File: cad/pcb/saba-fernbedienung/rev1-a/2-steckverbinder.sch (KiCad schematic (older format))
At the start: 28 parts, among them J301 Conn_01x04, J302 Conn_01x04, J303 Micro_SD_Card, J304 Conn_01x04, J305 AudioJack3_Ground, J306 Conn_01x02, J307 Conn_01x04, J308 Conn_01x01, J309 Conn_01x01, J310 Conn_01x01, J311 Conn_01x04, J312 USB_C_Receptacle_USB2.0, U301 TSOP31238

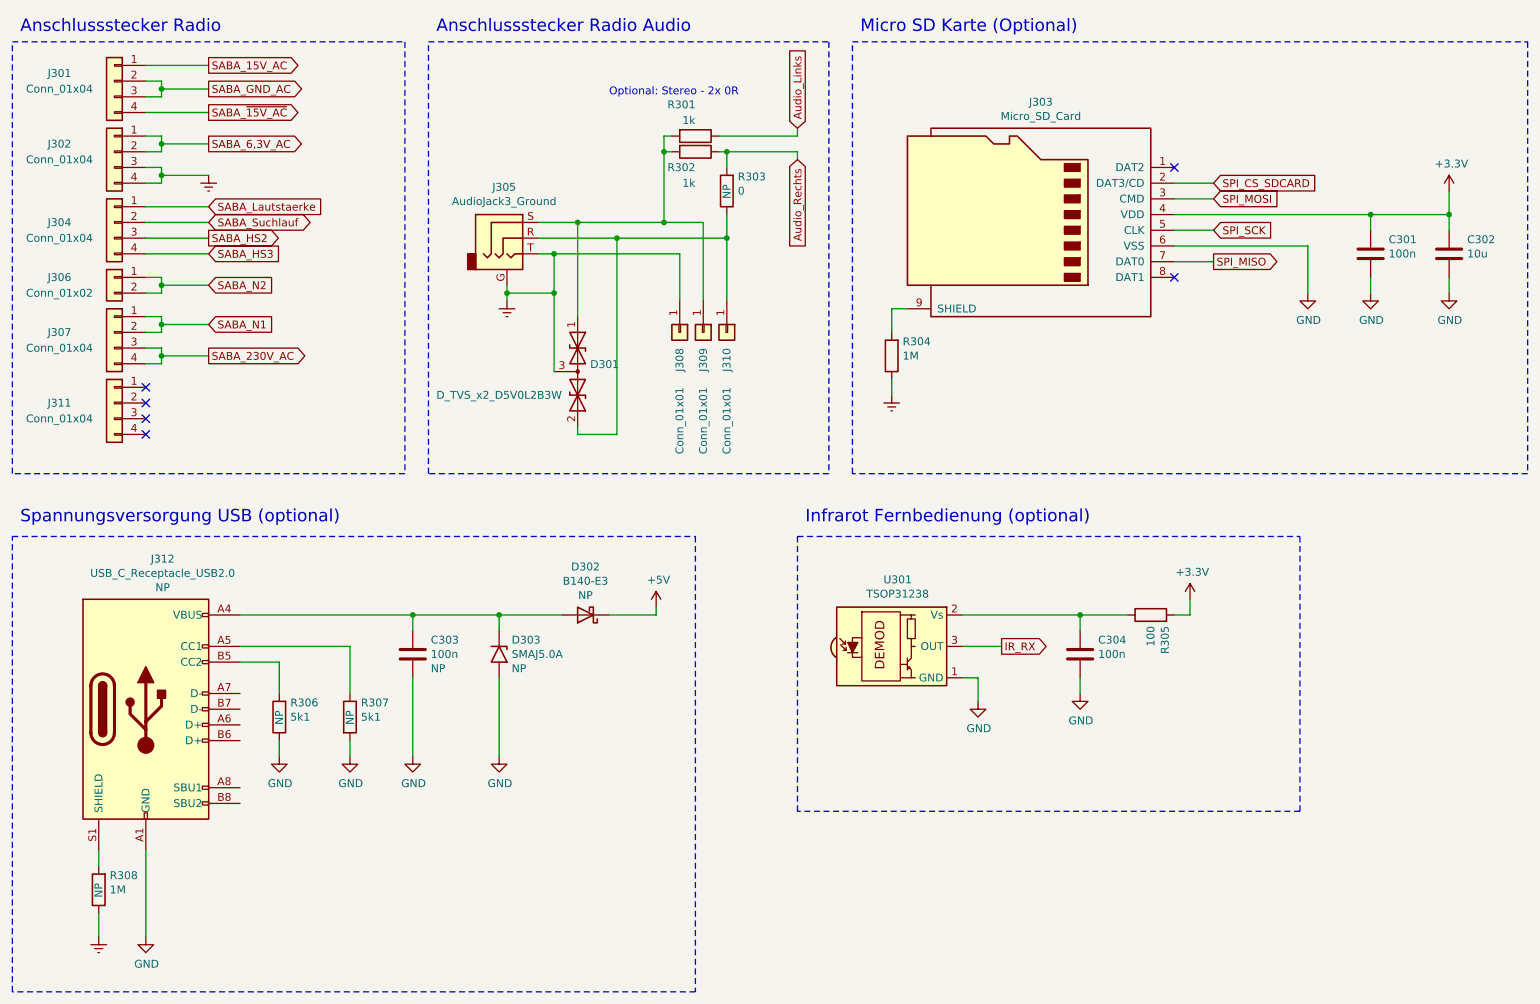
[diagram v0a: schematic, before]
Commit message: Fix: Div. DRC
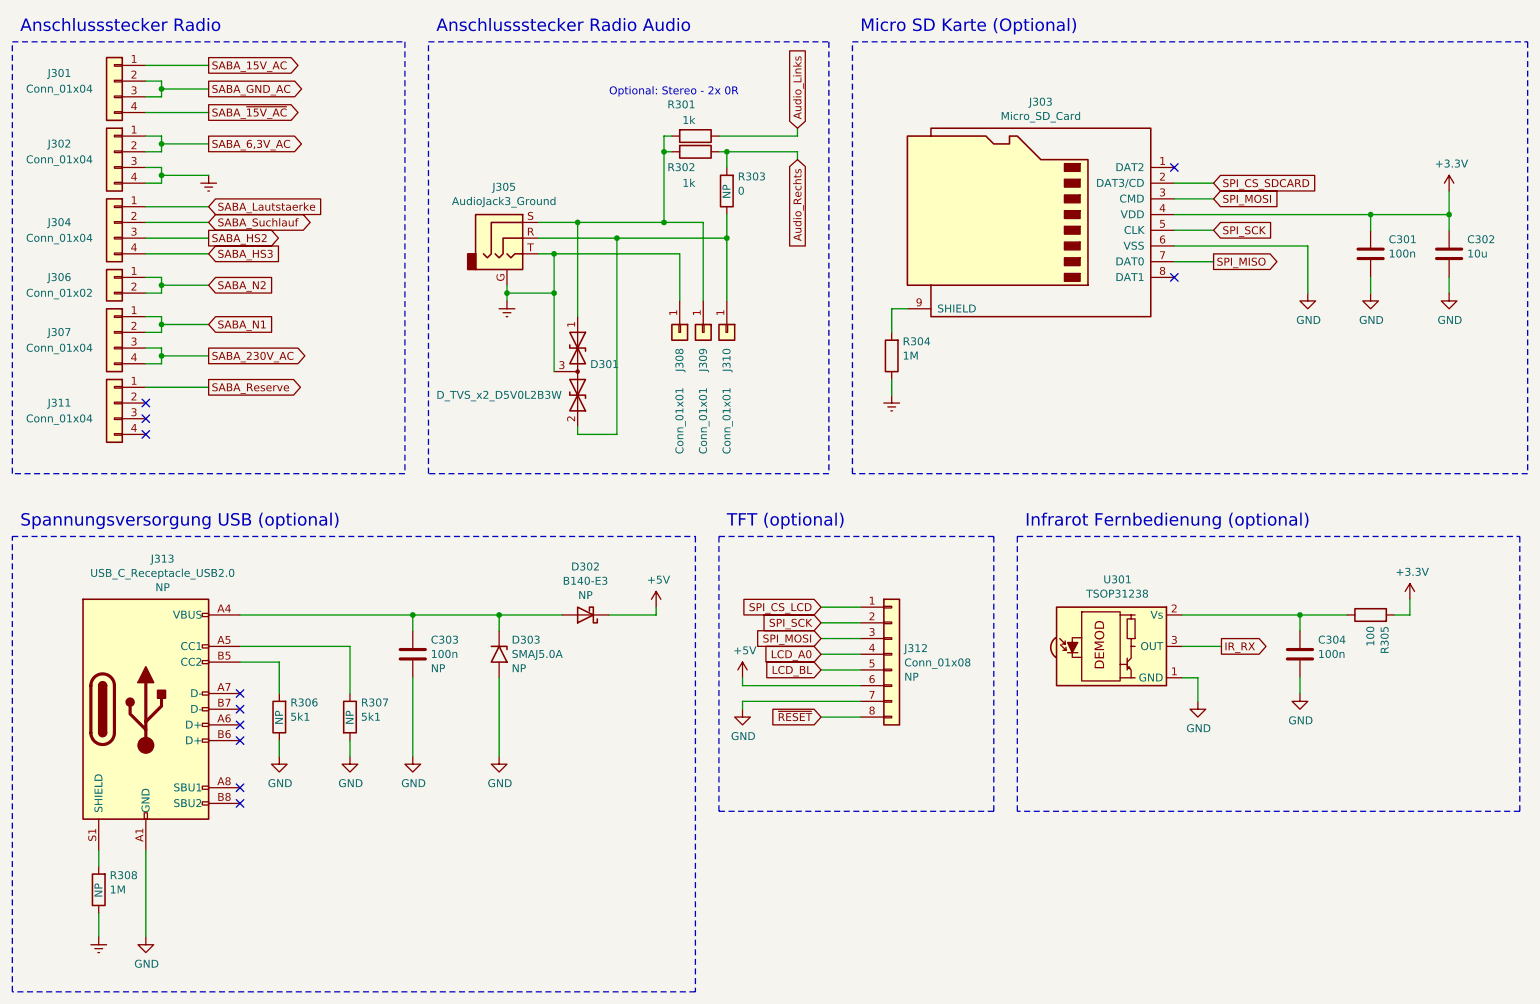
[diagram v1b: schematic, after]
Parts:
- added J312: Conn_01x08, symbol Connector_Generic:Conn_01x08
- renumbered J312 to J313
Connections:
- net +5V: now also J312.6 (Pin_6)
- net GND: now also J312.7 (Pin_7)
- net SPI_MOSI: now also J312.3 (Pin_3)
- net SPI_SCK: now also J312.2 (Pin_2)
- net SABA_Reserve: now reaches J311.1 (Pin_1)
- new net LCD_A0: J312.4 (Pin_4)
- new net LCD_BL: J312.5 (Pin_5)
- new net SPI_CS_LCD: J312.1 (Pin_1)
- new net ~RESET: J312.8 (Pin_8)
- no-connect marks 6 -> 11
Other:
- note added: "Infrarot Fernbedienung (optional)"
- note added: "Spannungsversorgung USB (optional)"
- note added: "TFT (optional)"
- note removed: "Infrarot Fernbedienung (optional)\n\n"
- note removed: "Spannungsversorgung USB (optional)\n\n"
- moved on the sheet: C304, R305, U301
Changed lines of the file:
@@
 	1950 3050 1850 3050
 Connection ~ 1950 3000
-NoConn ~ 1850 3200
 NoConn ~ 1850 3300
 NoConn ~ 1850 3400
@@
 Anschlussstecker Radio
 $Comp
-L Connector:USB_C_Receptacle_USB2.0 J312
+L Connector:USB_C_Receptacle_USB2.0 J313
 U 1 1 6005055F
 P 1850 5250
-F 0 "J312" H 1957 6207 50  0000 C CNN
+F 0 "J313" H 1957 6207 50  0000 C CNN
 F 1 "USB_C_Receptacle_USB2.0" H 1957 6116 50  0000 C CNN
 F 2 "" H 2000 5250 50  0001 C CNN
@@
 Wire Notes Line
 	1000 7050 1000 4150
-Text Notes 1050 4200 0    79   ~ 0
-Spannungsversorgung USB (optional)\n\n
-$Comp
-L power:GND #PWR0317
+Text Notes 1050 4100 0    79   ~ 0
+Spannungsversorgung USB (optional)
+$Comp
+L power:GND #PWR0319
 U 1 1 60063A29
 P 1850 6700
-F 0 "#PWR0317" H 1850 6450 50  0001 C CNN
+F 0 "#PWR0319" H 1850 6450 50  0001 C CNN
 F 1 "GND" H 1855 6527 50  0000 C CNN
 F 2 "" H 1850 6700 50  0001 C CNN
@@
 	2450 4950 2700 4950
 $Comp
-L power:GND #PWR0313
+L power:GND #PWR0315
 U 1 1 6006013B
 P 3150 5550
-F 0 "#PWR0313" H 3150 5300 50  0001 C CNN
+F 0 "#PWR0315" H 3150 5300 50  0001 C CNN
 F 1 "GND" H 3155 5377 50  0000 C CNN
 F 2 "" H 3150 5550 50  0001 C CNN
@@
 $EndComp
 $Comp
-L power:GND #PWR0312
+L power:GND #PWR0314
 U 1 1 6005FCD0
 P 2700 5550
-F 0 "#PWR0312" H 2700 5300 50  0001 C CNN
+F 0 "#PWR0314" H 2700 5300 50  0001 C CNN
 F 1 "GND" H 2705 5377 50  0000 C CNN
 F 2 "" H 2700 5550 50  0001 C CNN
@@
 	2450 4650 3550 4650
 $Comp
-L power:GND #PWR0314
+L power:GND #PWR0316
 U 1 1 600712E7
 P 3550 5550
-F 0 "#PWR0314" H 3550 5300 50  0001 C CNN
+F 0 "#PWR0316" H 3550 5300 50  0001 C CNN
 F 1 "GND" H 3555 5377 50  0000 C CNN
 F 2 "" H 3550 5550 50  0001 C CNN
@@
 $EndComp
 $Comp
-L power:GND #PWR0315
+L power:GND #PWR0317
 U 1 1 6007D5DC
 P 4100 5550
-F 0 "#PWR0315" H 4100 5300 50  0001 C CNN
+F 0 "#PWR0317" H 4100 5300 50  0001 C CNN
 F 1 "GND" H 4105 5377 50  0000 C CNN
 F 2 "" H 4100 5550 50  0001 C CNN
@@
 L Interface_Optical:TSOP312xx U301
 U 1 1 60019665
-P 6650 4850
-F 0 "U301" H 6638 5275 50  0000 C CNN
-F 1 "TSOP31238" H 6638 5184 50  0000 C CNN
-F 2 "OptoDevice:Vishay_CAST-3Pin" H 6600 4475 50  0001 C CNN
-F 3 "http://www.vishay.com/docs/82492/tsop312.pdf" H 7300 5150 50  0001 C CNN
-	1    6650 4850
-	1    0    0    -1
-$EndComp
-$Comp
-L power:GND #PWR0311
+P 8050 4850
+F 0 "U301" H 8038 5275 50  0000 C CNN
+F 1 "TSOP31238" H 8038 5184 50  0000 C CNN
+F 2 "OptoDevice:Vishay_CAST-3Pin" H 8000 4475 50  0001 C CNN
+F 3 "http://www.vishay.com/docs/82492/tsop312.pdf" H 8700 5150 50  0001 C CNN
+	1    8050 4850
+	1    0    0    -1
+$EndComp
+$Comp
+L power:GND #PWR0312
 U 1 1 6001F94B
-P 7150 5200
-F 0 "#PWR0311" H 7150 4950 50  0001 C CNN
-F 1 "GND" H 7155 5027 50  0000 C CNN
-F 2 "" H 7150 5200 50  0001 C CNN
-F 3 "" H 7150 5200 50  0001 C CNN
-	1    7150 5200
-	1    0    0    -1
-$EndComp
-Text GLabel 7300 4850 2    50   Output ~ 0
+P 8550 5200
+F 0 "#PWR0312" H 8550 4950 50  0001 C CNN
+F 1 "GND" H 8555 5027 50  0000 C CNN
+F 2 "" H 8550 5200 50  0001 C CNN
+F 3 "" H 8550 5200 50  0001 C CNN
+	1    8550 5200
+	1    0    0    -1
+$EndComp
+Text GLabel 8700 4850 2    50   Output ~ 0
 IR_RX
 Wire Wire Line
-	7050 4850 7300 4850
-Wire Wire Line
-	7050 5050 7150 5050
-Wire Wire Line
-	7150 5050 7150 5200
-Wire Notes Line
-	6000 4150 9200 4150
-Wire Notes Line
-	9200 4150 9200 5900
-Wire Notes Line
-	9200 5900 6000 5900
-Wire Notes Line
-	6000 5900 6000 4150
-Text Notes 6050 4200 0    79   ~ 0
-Infrarot Fernbedienung (optional)\n\n
+	8450 4850 8700 4850
+Wire Wire Line
+	8450 5050 8550 5050
+Wire Wire Line
+	8550 5050 8550 5200
+Wire Notes Line
+	7400 4150 10600 4150
+Wire Notes Line
+	10600 4150 10600 5900
+Wire Notes Line
+	10600 5900 7400 5900
+Wire Notes Line
+	7400 5900 7400 4150
+Text Notes 7450 4100 0    79   ~ 0
+Infrarot Fernbedienung (optional)
 $Comp
 L Connector:AudioJack3_Ground J305
@@
 Connection ~ 4450 2350
 Wire Wire Line
-	7800 4650 7050 4650
-Wire Wire Line
-	7800 4750 7800 4650
-Wire Wire Line
-	7800 5150 7800 5050
-Connection ~ 7800 4650
-Wire Wire Line
-	8100 4650 7800 4650
-Wire Wire Line
-	8500 4650 8400 4650
-Wire Wire Line
-	8500 4550 8500 4650
+	9200 4650 8450 4650
+Wire Wire Line
+	9200 4750 9200 4650
+Wire Wire Line
+	9200 5150 9200 5050
+Connection ~ 9200 4650
+Wire Wire Line
+	9500 4650 9200 4650
+Wire Wire Line
+	9900 4650 9800 4650
+Wire Wire Line
+	9900 4550 9900 4650
 $Comp
 L power:+3.3V #PWR0308
 U 1 1 60021397
-P 8500 4550
-F 0 "#PWR0308" H 8500 4400 50  0001 C CNN
-F 1 "+3.3V" H 8515 4723 50  0000 C CNN
-F 2 "" H 8500 4550 50  0001 C CNN
-F 3 "" H 8500 4550 50  0001 C CNN
-	1    8500 4550
-	1    0    0    -1
-$EndComp
-$Comp
-L power:GND #PWR0310
+P 9900 4550
+F 0 "#PWR0308" H 9900 4400 50  0001 C CNN
+F 1 "+3.3V" H 9915 4723 50  0000 C CNN
+F 2 "" H 9900 4550 50  0001 C CNN
+F 3 "" H 9900 4550 50  0001 C CNN
+	1    9900 4550
+	1    0    0    -1
+$EndComp
+$Comp
+L power:GND #PWR0311
 U 1 1 60020161
-P 7800 5150
-F 0 "#PWR0310" H 7800 4900 50  0001 C CNN
-F 1 "GND" H 7805 4977 50  0000 C CNN
-F 2 "" H 7800 5150 50  0001 C CNN
-F 3 "" H 7800 5150 50  0001 C CNN
-	1    7800 5150
+P 9200 5150
+F 0 "#PWR0311" H 9200 4900 50  0001 C CNN
+F 1 "GND" H 9205 4977 50  0000 C CNN
+F 2 "" H 9200 5150 50  0001 C CNN
+F 3 "" H 9200 5150 50  0001 C CNN
+	1    9200 5150
 	1    0    0    -1
 $EndComp
@@
 L Device:C C304
 U 1 1 6001EC41
-P 7800 4900
-F 0 "C304" H 7915 4991 50  0000 L CNN
-F 1 "100n" H 7915 4900 50  0000 L CNN
-F 2 "Capacitor_SMD:C_0603_1608Metric" H 7838 4750 50  0001 C CNN
-F 3 "~" H 7800 4900 50  0001 C CNN
-F 4 "" H 7915 4809 50  0000 L CNN "Placement"
-	1    7800 4900
+P 9200 4900
+F 0 "C304" H 9315 4991 50  0000 L CNN
+F 1 "100n" H 9315 4900 50  0000 L CNN
+F 2 "Capacitor_SMD:C_0603_1608Metric" H 9238 4750 50  0001 C CNN
+F 3 "~" H 9200 4900 50  0001 C CNN
+F 4 "" H 9315 4809 50  0000 L CNN "Placement"
+	1    9200 4900
 	1    0    0    -1
 $EndComp
@@
 L Device:R R?
 U 1 1 6001BDE1
-P 8250 4650
+P 9650 4650
 AR Path="/5FFC49DA/6001BDE1" Ref="R?"  Part="1"
 AR Path="/6002EA57/6001BDE1" Ref="R305"  Part="1"
-F 0 "R305" H 8180 4559 50  0000 R CNN
-F 1 "100" H 8180 4650 50  0000 R CNN
-F 2 "Resistor_SMD:R_0603_1608Metric" V 8180 4650 50  0001 C CNN
-F 3 "~" H 8250 4650 50  0001 C CNN
-F 4 "" V 8250 4700 50  0000 R CNN "Placement"
-	1    8250 4650
+F 0 "R305" H 9580 4559 50  0000 R CNN
+F 1 "100" H 9580 4650 50  0000 R CNN
+F 2 "Resistor_SMD:R_0603_1608Metric" V 9580 4650 50  0001 C CNN
+F 3 "~" H 9650 4650 50  0001 C CNN
+F 4 "" V 9650 4700 50  0000 R CNN "Placement"
+	1    9650 4650
 	0    -1   -1   0
 $EndComp
@@
 $EndComp
 $Comp
-L power:Earth #PWR0316
+L power:Earth #PWR0318
 U 1 1 600AE860
 P 1550 6700
-F 0 "#PWR0316" H 1550 6450 50  0001 C CNN
+F 0 "#PWR0318" H 1550 6450 50  0001 C CNN
 F 1 "Earth" H 1550 6550 50  0001 C CNN
 F 2 "" H 1550 6700 50  0001 C CNN
@@
 	4450 3100 4450 2600
 Connection ~ 4450 2600
+Text GLabel 2250 3200 2    50   Output ~ 0
+SABA_Reserve
+Wire Wire Line
+	2250 3200 1850 3200
+$Comp
+L Connector_Generic:Conn_01x08 J312
+U 1 1 60A4DF30
+P 6600 4900
+F 0 "J312" H 6680 4937 50  0000 L CNN
+F 1 "Conn_01x08" H 6680 4846 50  0000 L CNN
+F 2 "" H 6600 4900 50  0001 C CNN
+F 3 "~" H 6600 4900 50  0001 C CNN
+F 4 "NP" H 6680 4755 50  0000 L CNN "Placement"
+	1    6600 4900
+	1    0    0    -1
+$EndComp
+Text GLabel 6150 4600 0    50   Input ~ 0
+SPI_CS_LCD
+Text GLabel 6150 4700 0    50   Input ~ 0
+SPI_SCK
+Text GLabel 6150 4800 0    50   Input ~ 0
+SPI_MOSI
+Text GLabel 6150 5300 0    50   Input ~ 0
+~RESET
+Text GLabel 6150 4900 0    50   Input ~ 0
+LCD_A0
+Text GLabel 6150 5000 0    50   Input ~ 0
+LCD_BL
+$Comp
+L power:+5V #PWR0310
+U 1 1 60A526F1
+P 5650 5050
+F 0 "#PWR0310" H 5650 4900 50  0001 C CNN
+F 1 "+5V" H 5665 5223 50  0000 C CNN
+F 2 "" H 5650 5050 50  0001 C CNN
+F 3 "" H 5650 5050 50  0001 C CNN
+	1    5650 5050
+	1    0    0    -1
+$EndComp
+$Comp
+L power:GND #PWR0313
+U 1 1 60A52FFC
+P 5650 5250
+F 0 "#PWR0313" H 5650 5000 50  0001 C CNN
+F 1 "GND" H 5655 5077 50  0000 C CNN
+F 2 "" H 5650 5250 50  0001 C CNN
+F 3 "" H 5650 5250 50  0001 C CNN
+	1    5650 5250
+	1    0    0    -1
+$EndComp
+Wire Wire Line
+	6150 4600 6400 4600
+Wire Wire Line
+	6150 4700 6400 4700
+Wire Wire Line
+	6150 4800 6400 4800
+Wire Wire Line
+	6150 4900 6400 4900
+Wire Wire Line
+	6400 5000 6150 5000
+Wire Wire Line
+	6400 5100 5650 5100
+Wire Wire Line
+	5650 5100 5650 5050
+Wire Wire Line
+	6400 5200 5650 5200
+Wire Wire Line
+	5650 5200 5650 5250
+Wire Wire Line
+	6400 5300 6150 5300
+Text Notes 5550 4100 0    79   ~ 0
+TFT (optional)
+Wire Notes Line
+	5500 4150 7250 4150
+Wire Notes Line
+	7250 4150 7250 5900
+Wire Notes Line
+	7250 5900 5500 5900
+Wire Notes Line
+	5500 5900 5500 4150
+NoConn ~ 2450 5150
+NoConn ~ 2450 5250
+NoConn ~ 2450 5350
+NoConn ~ 2450 5450
+NoConn ~ 2450 5750
+NoConn ~ 2450 5850
 $EndSCHEMATC
